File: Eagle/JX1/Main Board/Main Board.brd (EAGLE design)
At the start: 50.8 x 76.2 mm, 9 parts, among them J1 RASPBERRYPI-40-PIN-GPIO_PTH_N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, U1 SN74HC595N, U2 SN74HC595N

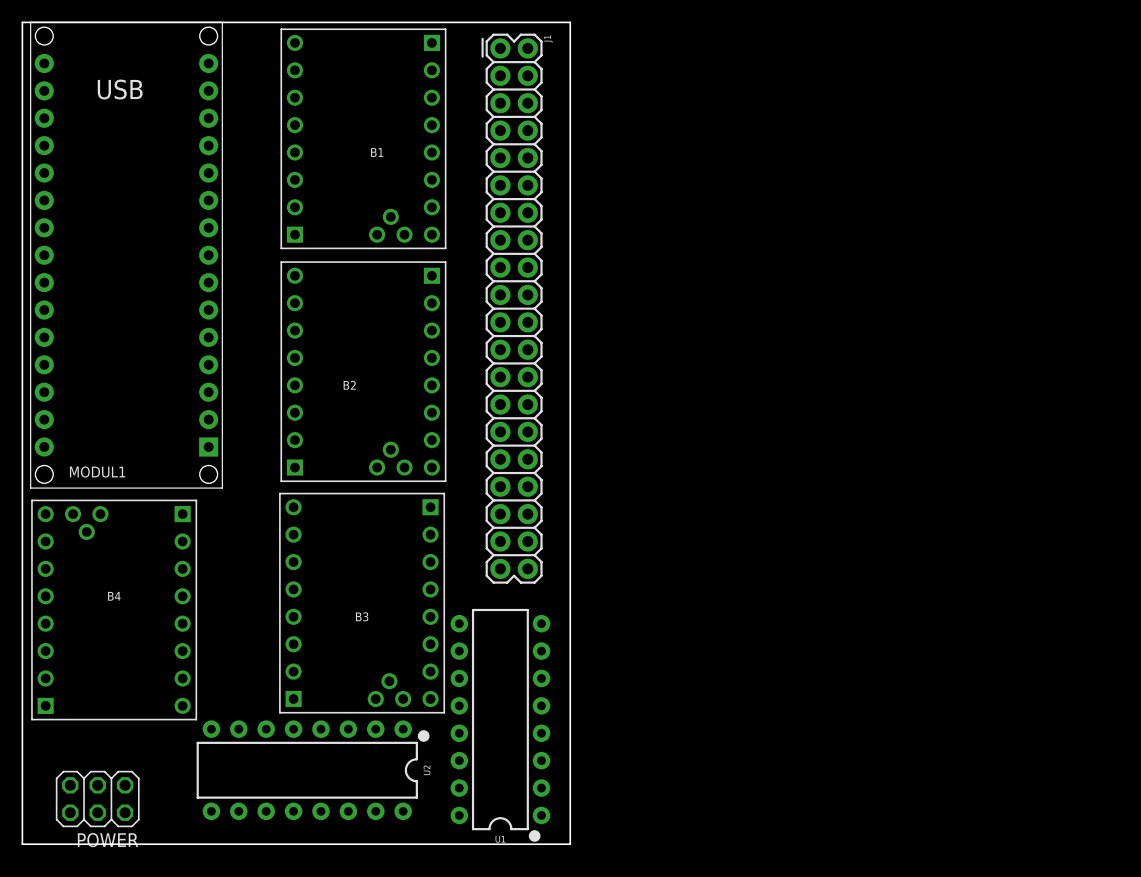
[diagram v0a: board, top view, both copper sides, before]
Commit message: More board Changes
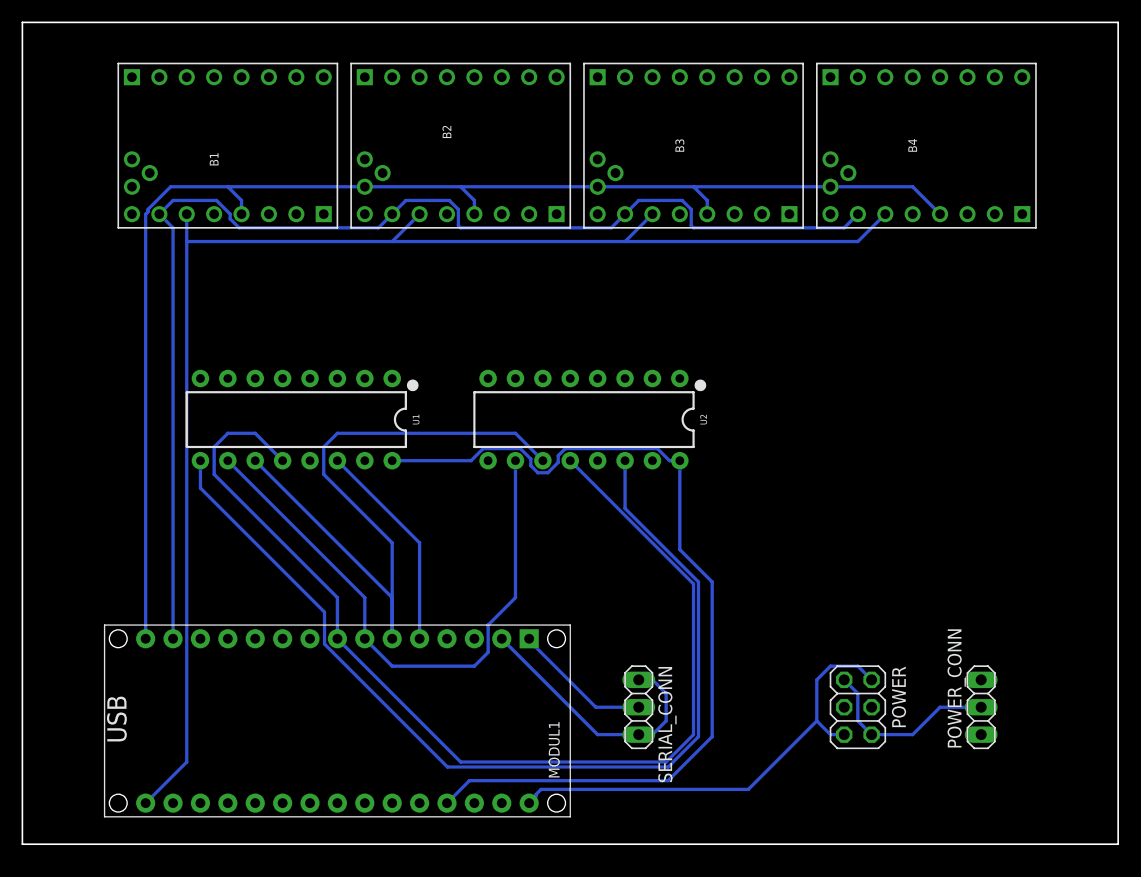
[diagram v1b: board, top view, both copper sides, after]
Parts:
- removed J1: RASPBERRYPI-40-PIN-GPIO_PTH_NO_SHROUD, SparkFun-Connectors:2X20
- added POWER_CONN, SERIAL_CONN: (no value), pinhead:1X03
- moved B4 86.7 mm to (83.8, 64.8), turned to 90 degrees
- moved POWER 71.0 mm to (77.5, 12.7), turned to 270 degrees
- moved B3 52.4 mm to (62.2, 64.8), turned to 90 degrees
- moved MODUL1 47.4 mm to (29.2, 11.4), turned to 270 degrees
- moved U2 41.4 mm to (52.1, 39.4)
- moved U1 33.6 mm to (25.4, 39.4), turned to 180 degrees
- moved B2 22.8 mm to (40.6, 64.8), turned to 90 degrees
- moved B1 12.6 mm to (19.1, 64.8), turned to 90 degrees
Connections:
- net N$19 renamed SCK
- net N$20 renamed MOSI
- net N$21 renamed MISO
- net N$23 renamed SSCK
- net N$24 renamed SCL
- net N$25 renamed RCK
- removed net 3.3V: J1.1, J1.17
- removed net N$26: J1.10, MODUL1.J1.1
- new net N$1: MODUL1.J1.1, SERIAL_CONN.2
- net +5V: now also POWER_CONN.2; no longer J1.2, J1.4
- net GND: now also POWER_CONN.1, POWER_CONN.3; no longer J1.14, J1.20, J1.25, J1.30, J1.34, J1.39, J1.6, J1.9
- net N$27: now also SERIAL_CONN.1, SERIAL_CONN.3; no longer J1.8
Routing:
- net SCK: track 0.00 -> 129.2 mm
- net MISO: track 0.00 -> 124.5 mm
- net MOSI: track 0.00 -> 113.0 mm
- net +5V: track 0.00 -> 101.5 mm
- net RCK: track 0.00 -> 99.4 mm
- net N$2: track 0.00 -> 90.7 mm
- net SSCK: track 0.00 -> 64.1 mm
- net SCL: track 0.00 -> 53.6 mm
- net +12V: track 0.00 -> 42.9 mm
- net N$27: track 0.00 -> 25.1 mm
- net N$22: track 0.00 -> 19.7 mm
- net N$1: track 0.00 -> 12.9 mm
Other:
- board size 50.8 x 76.2 mm -> 101.6 x 76.2 mm
